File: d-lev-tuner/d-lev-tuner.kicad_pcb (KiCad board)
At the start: 4 copper layers, 88.7 x 68.4 mm, 38 parts, among them J1 S6B-PH-SM4-TB, U1 STP08CP05, U2 STP08CP05, U3 AP2112K-3.3, U4 STP08CP05, U5 DSM7TA56

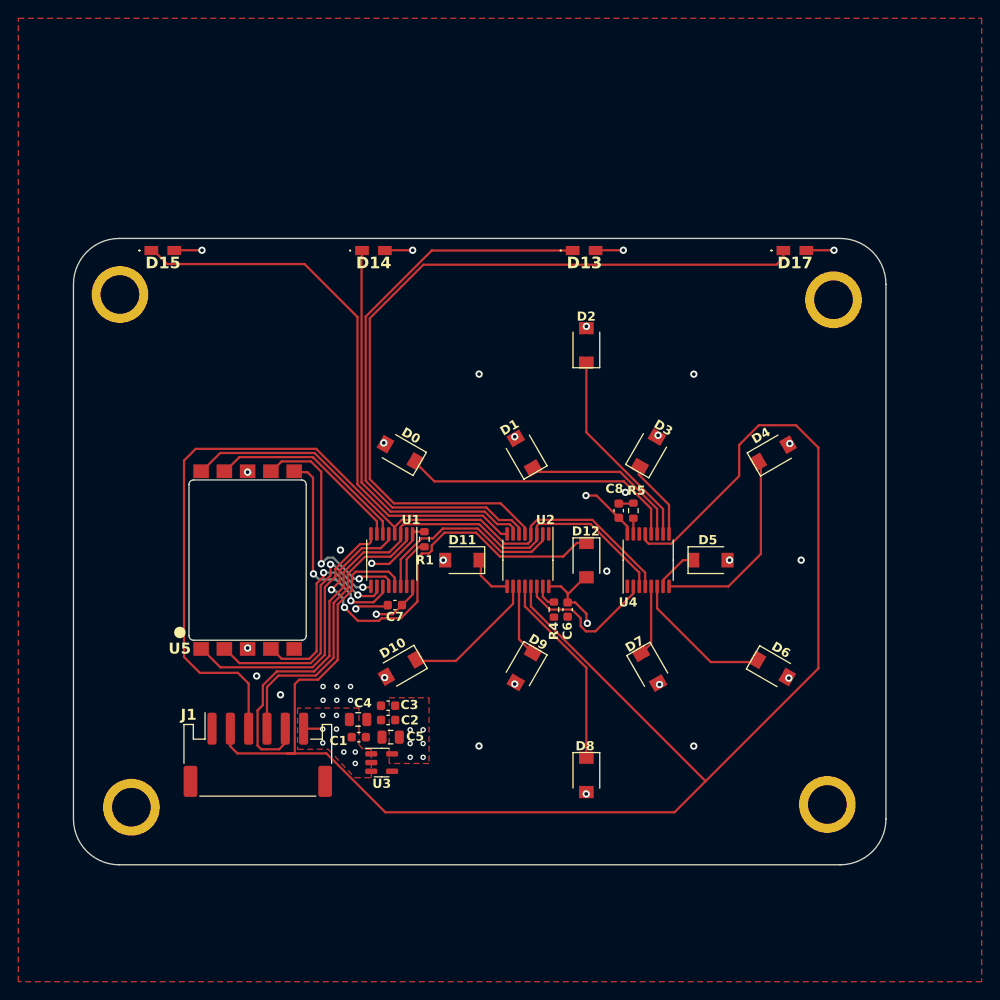
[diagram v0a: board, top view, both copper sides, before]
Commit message: star pattern done
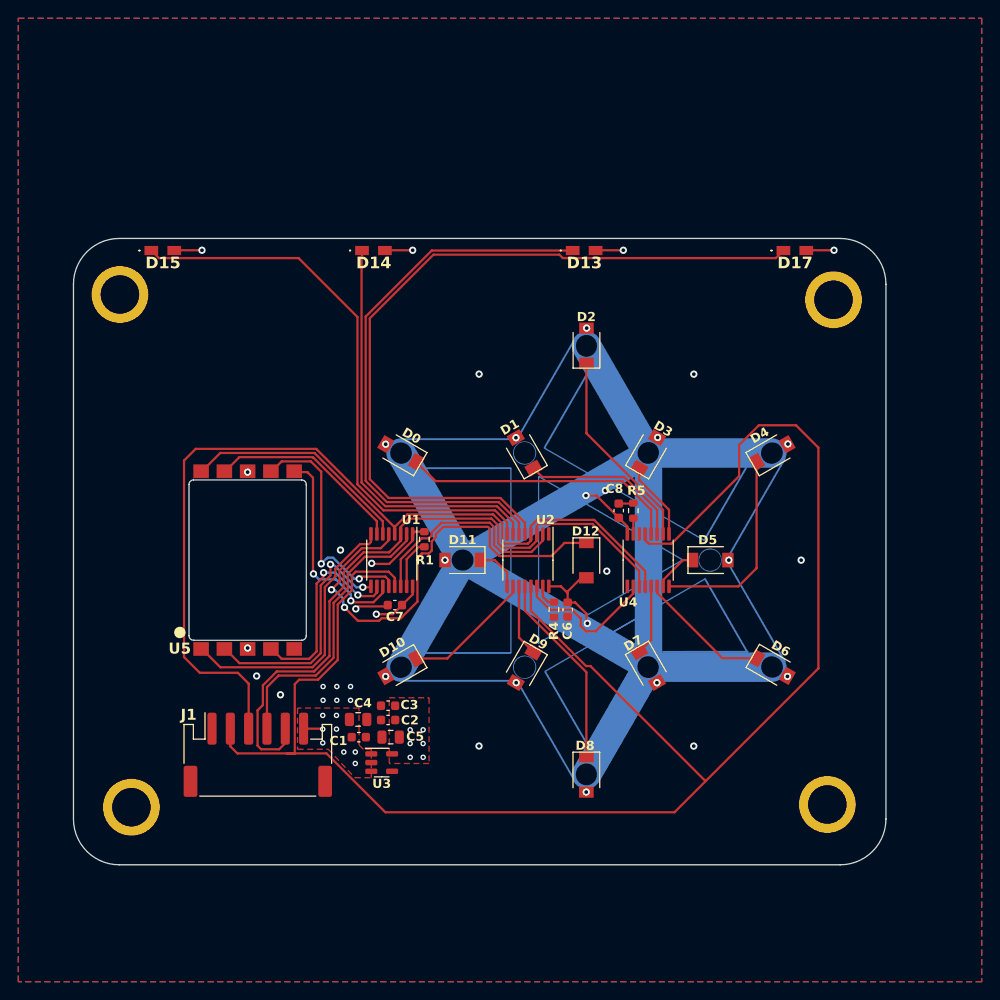
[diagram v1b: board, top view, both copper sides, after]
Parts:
- added REF**: star-pattern, art:star-pattern, B.Cu at (100.2, 66.4)
- moved D7 0.19 mm to (106.9, 78.1)
- moved D6 0.16 mm to (120.4, 78.1)
- moved D4 0.14 mm to (120.4, 54.7)
- moved D3 0.12 mm to (106.9, 54.7)
- moved D10 0.09 mm to (79.9, 78.1)
- moved D0 0.07 mm to (79.9, 54.7)
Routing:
- net LED12: track 48.4 -> 50.5 mm
- net /Net-(U3-SDI): track 22.1 -> 24.0 mm
- net CLK: track 72.4 -> 74.1 mm
- net LE: track 97.8 -> 99.6 mm
- net LED4: track 20.9 -> 22.0 mm
- net LED6: track 15.3 -> 14.5 mm
- net LED16: track 62.4 -> 63.1 mm
- net LED11: track 4.41 -> 5.01 mm
- net LED9: track 7.24 -> 7.82 mm
- net LED7: track 7.13 -> 7.69 mm
- added copper zone on B.Cu, net GND
